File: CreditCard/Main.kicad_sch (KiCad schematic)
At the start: 28 parts, among them J2 LCD, SW1 2425754-1, SW2 2425754-1, SW3 2425754-1, U10 PAM8403DR, U11 SPKM.36.8.B, U5 PTS645SK43SMTR92LFS, U6 PTS645SK43SMTR92LFS, U7 PTS645SK43SMTR92LFS, U9 SPKM.36.8.B

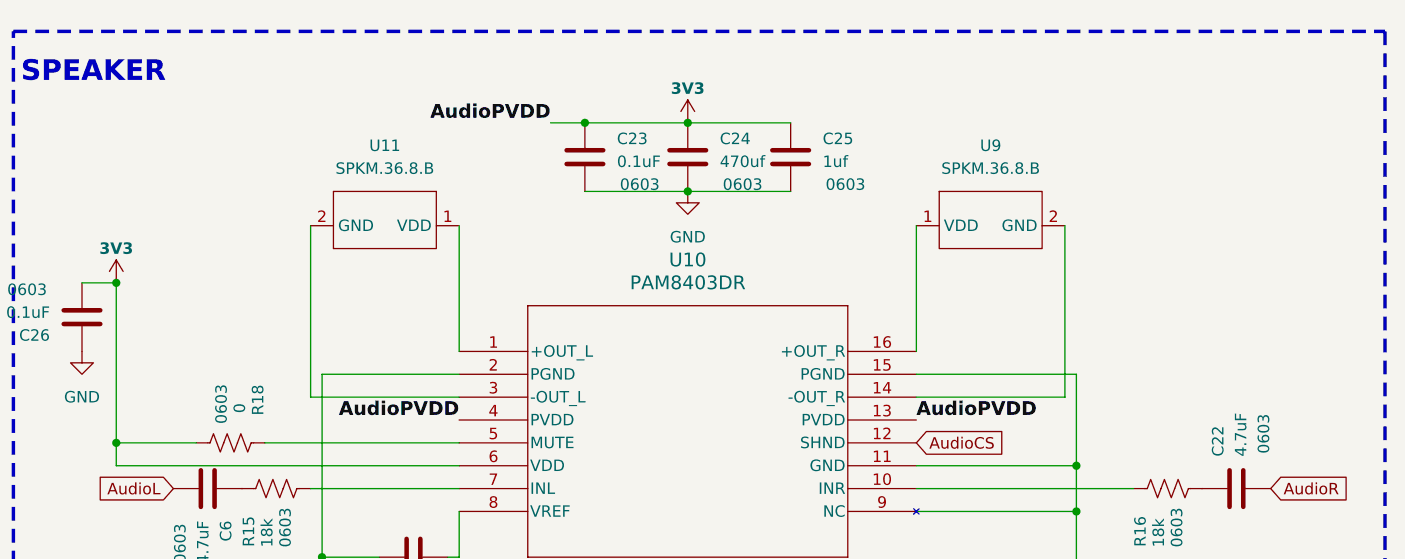
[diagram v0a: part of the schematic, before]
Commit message: petite retouche et bom complet
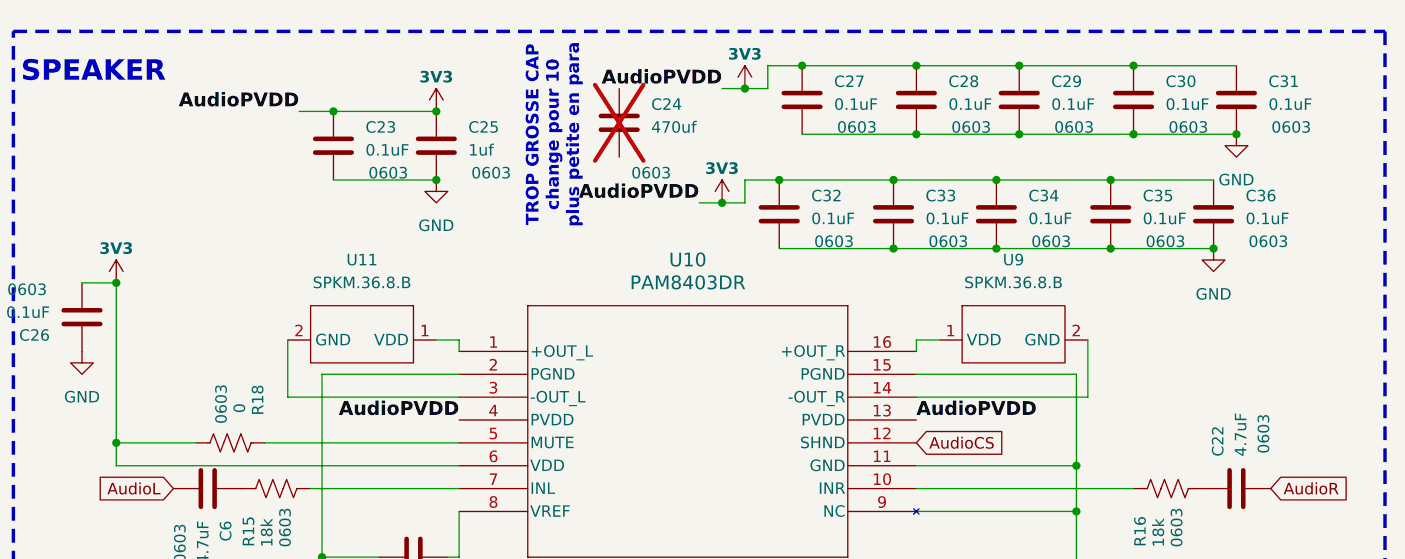
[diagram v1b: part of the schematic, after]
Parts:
- added C27, C28, C29, C30, C31, C32, C33, C34, C35, C36: 0.1uF, Capacitor_SMD:C_0603_1608Metric, symbol Device:C
- C24: now not fitted; now left out of the parts list
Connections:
- net 3V3: now also C27.1, C28.1, C29.1, C30.1, C31.1, C32.1, C33.1, C34.1, C35.1, C36.1; no longer C24.1
- net GND: now also C27.2, C28.2, C29.2, C30.2, C31.2, C32.2, C33.2, C34.2, C35.2, C36.2; no longer C24.2
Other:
- note added: "TROP GROSSE CAP change pour 10 plus petite en para"
- moved on the sheet: C23, C25, U11, U9
